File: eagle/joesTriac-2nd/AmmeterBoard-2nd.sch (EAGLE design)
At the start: 34 parts, among them IC2 TLC251P, IC3 TLC251_or_311, IC4 INA118P, IC5 TLC251_or_311, IC6 TLC251P, IC7 ACS758ECB-200B-PFF-T, T1 2N3441, X1 1, X2 2, X6 1751264

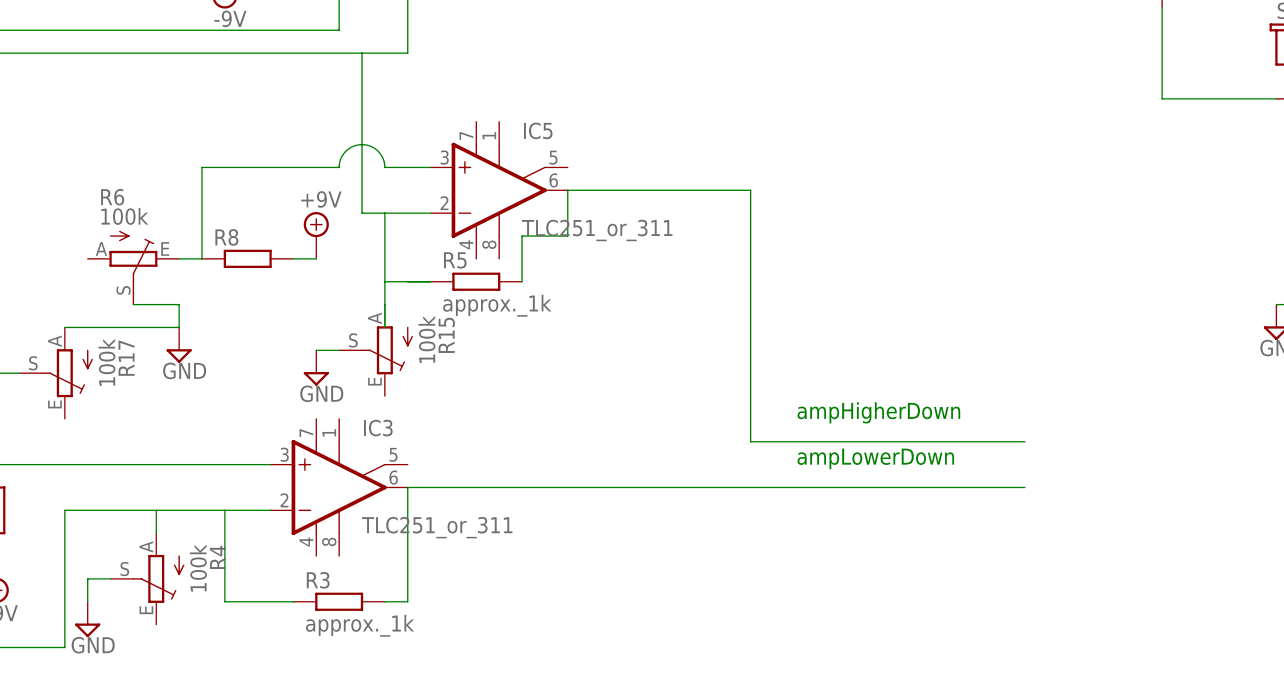
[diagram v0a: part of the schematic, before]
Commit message: reg save,ampsZeroPass tobe tested
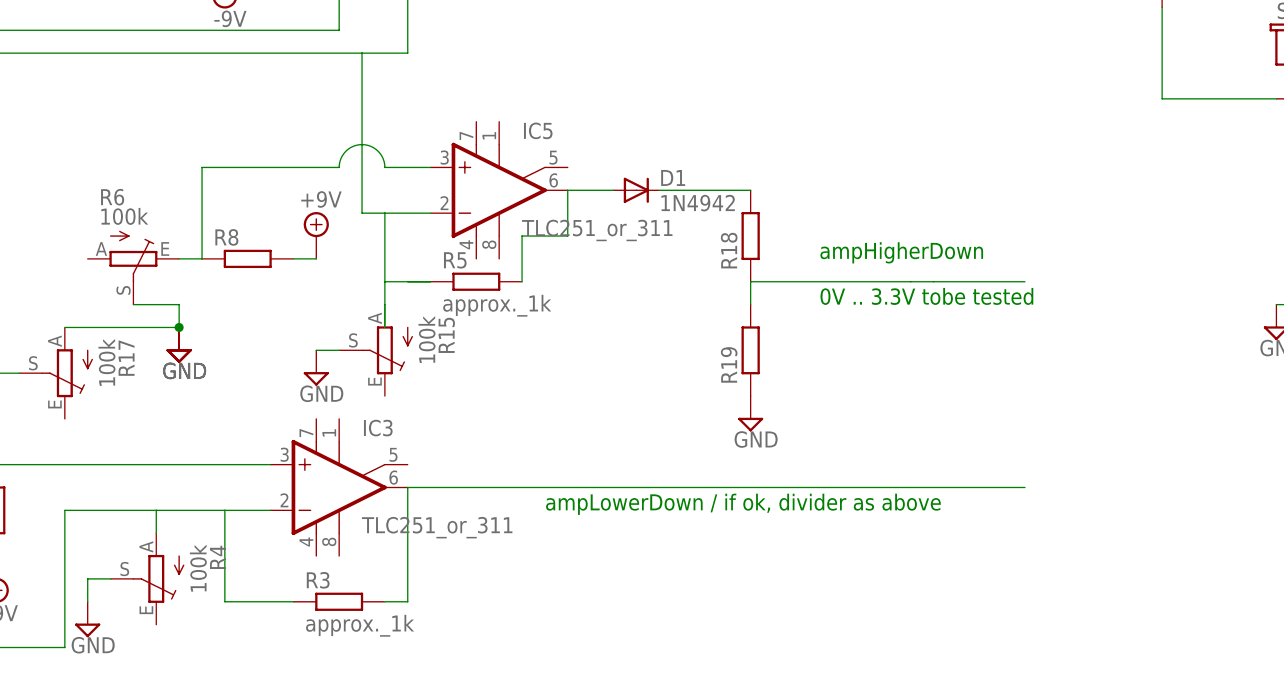
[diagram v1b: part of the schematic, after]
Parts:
- added D1: 1N4942, diode:1N4942
- added R18, R19: (no value), resistor:R-EU_0207/10
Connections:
- new net N$28: D1.A, IC5.OUT, R5.2
- new net N$29: D1.C, R18.2
- net GND: now also R19.1
- net N$30: now also R18.1, R19.2; no longer IC5.OUT, R5.2
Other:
- note added: "0V .. 3.3V tobe tested"
- note added: "ampLowerDown / if ok, divider as above"
- note removed: "ampLowerDown"
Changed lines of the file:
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@@
 <layer number="97" name="Info" color="7" fill="1" visible="yes" active="yes"/>
 <layer number="98" name="Guide" color="6" fill="1" visible="yes" active="yes"/>
+<layer number="99" name="SpiceOrder" color="5" fill="1" visible="yes" active="yes"/>
 <layer number="101" name="Hidden" color="15" fill="1" visible="yes" active="yes"/>
 <layer number="102" name="Changes" color="12" fill="1" visible="yes" active="yes"/>
@@
 <part name="SUPPLY8" library="supply2" deviceset="+9V" device=""/>
 <part name="SUPPLY28" library="supply2" deviceset="-9V" device=""/>
+<part name="D1" library="diode" deviceset="1N4942" device=""/>
+<part name="R18" library="resistor" deviceset="R-EU_" device="0207/10"/>
+<part name="R19" library="resistor" deviceset="R-EU_" device="0207/10"/>
+<part name="SUPPLY31" library="supply2" deviceset="GND" device=""/>
+<part name="SUPPLY32" library="supply2" deviceset="GND" device=""/>
 </parts>
 <sheets>
@@
 <text x="-17.78" y="109.22" size="2.54" layer="91">currentSensor</text>
 <text x="66.04" y="63.5" size="1.778" layer="91">WIP - work in progress in 637 part</text>
-<text x="88.9" y="-20.32" size="1.778" layer="91">ampHigherDown</text>
-<text x="88.9" y="-25.4" size="1.778" layer="91">ampLowerDown</text>
+<text x="91.44" y="-2.54" size="1.778" layer="91">ampHigherDown</text>
+<text x="60.96" y="-30.48" size="1.778" layer="91">ampLowerDown / if ok, divider as above</text>
 <text x="139.7" y="58.42" size="1.778" layer="91">ventually aplifier can be ommitted</text>
+<text x="91.44" y="-7.62" size="1.778" layer="91">0V .. 3.3V tobe tested</text>
 </plain>
 <instances>
@@
 <instance part="SUPPLY8" gate="G$1" x="35.56" y="0"/>
 <instance part="SUPPLY28" gate="G$1" x="0" y="-38.1"/>
+<instance part="D1" gate="1" x="71.12" y="5.08"/>
+<instance part="R18" gate="G$1" x="83.82" y="0" rot="R90"/>
+<instance part="R19" gate="G$1" x="83.82" y="-12.7" rot="R90"/>
+<instance part="SUPPLY31" gate="GND" x="20.32" y="-12.7"/>
+<instance part="SUPPLY32" gate="GND" x="83.82" y="-20.32"/>
 </instances>
 <busses>
@@
 <wire x1="15.24" y1="-7.62" x2="20.32" y2="-7.62" width="0.1524" layer="91"/>
 <wire x1="20.32" y1="-7.62" x2="20.32" y2="-10.16" width="0.1524" layer="91"/>
+<pinref part="SUPPLY31" gate="GND" pin="GND"/>
+<junction x="20.32" y="-10.16"/>
+</segment>
+<segment>
+<pinref part="R19" gate="G$1" pin="1"/>
+<pinref part="SUPPLY32" gate="GND" pin="GND"/>
 </segment>
 </net>
@@
 <wire x1="2.54" y1="-15.24" x2="0" y2="-15.24" width="0.1524" layer="91"/>
 <wire x1="0" y1="-15.24" x2="0" y2="-25.4" width="0.1524" layer="91"/>
-</segment>
-</net>
-<net name="N$30" class="0">
-<segment>
-<pinref part="R5" gate="G$1" pin="2"/>
-<wire x1="58.42" y1="-5.08" x2="58.42" y2="0" width="0.1524" layer="91"/>
-<pinref part="IC5" gate="A" pin="OUT"/>
-<wire x1="58.42" y1="0" x2="63.5" y2="0" width="0.1524" layer="91"/>
-<wire x1="63.5" y1="0" x2="63.5" y2="5.08" width="0.1524" layer="91"/>
-<wire x1="63.5" y1="5.08" x2="83.82" y2="5.08" width="0.1524" layer="91"/>
-<wire x1="83.82" y1="5.08" x2="83.82" y2="-22.86" width="0.1524" layer="91"/>
-<wire x1="83.82" y1="-22.86" x2="114.3" y2="-22.86" width="0.1524" layer="91"/>
 </segment>
 </net>
@@
 </segment>
 </net>
+<net name="N$28" class="0">
+<segment>
+<pinref part="IC5" gate="A" pin="OUT"/>
+<wire x1="63.5" y1="0" x2="63.5" y2="5.08" width="0.1524" layer="91"/>
+<wire x1="58.42" y1="0" x2="63.5" y2="0" width="0.1524" layer="91"/>
+<pinref part="R5" gate="G$1" pin="2"/>
+<wire x1="58.42" y1="-5.08" x2="58.42" y2="0" width="0.1524" layer="91"/>
+<pinref part="D1" gate="1" pin="A"/>
+<wire x1="63.5" y1="5.08" x2="68.58" y2="5.08" width="0.1524" layer="91"/>
+</segment>
+</net>
+<net name="N$29" class="0">
+<segment>
+<pinref part="D1" gate="1" pin="C"/>
+<wire x1="73.66" y1="5.08" x2="83.82" y2="5.08" width="0.1524" layer="91"/>
+<pinref part="R18" gate="G$1" pin="2"/>
+</segment>
+</net>
+<net name="N$30" class="0">
+<segment>
+<pinref part="R18" gate="G$1" pin="1"/>
+<pinref part="R19" gate="G$1" pin="2"/>
+<wire x1="83.82" y1="-5.08" x2="83.82" y2="-7.62" width="0.1524" layer="91"/>
+<wire x1="83.82" y1="-5.08" x2="101.6" y2="-5.08" width="0.1524" layer="91"/>
+<wire x1="114.3" y1="-5.08" x2="104.14" y2="-5.08" width="0.1524" layer="91"/>
+<wire x1="101.6" y1="-5.08" x2="104.14" y2="-5.08" width="0.1524" layer="91"/>
+</segment>
+</net>
